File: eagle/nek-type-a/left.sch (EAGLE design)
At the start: 68 parts

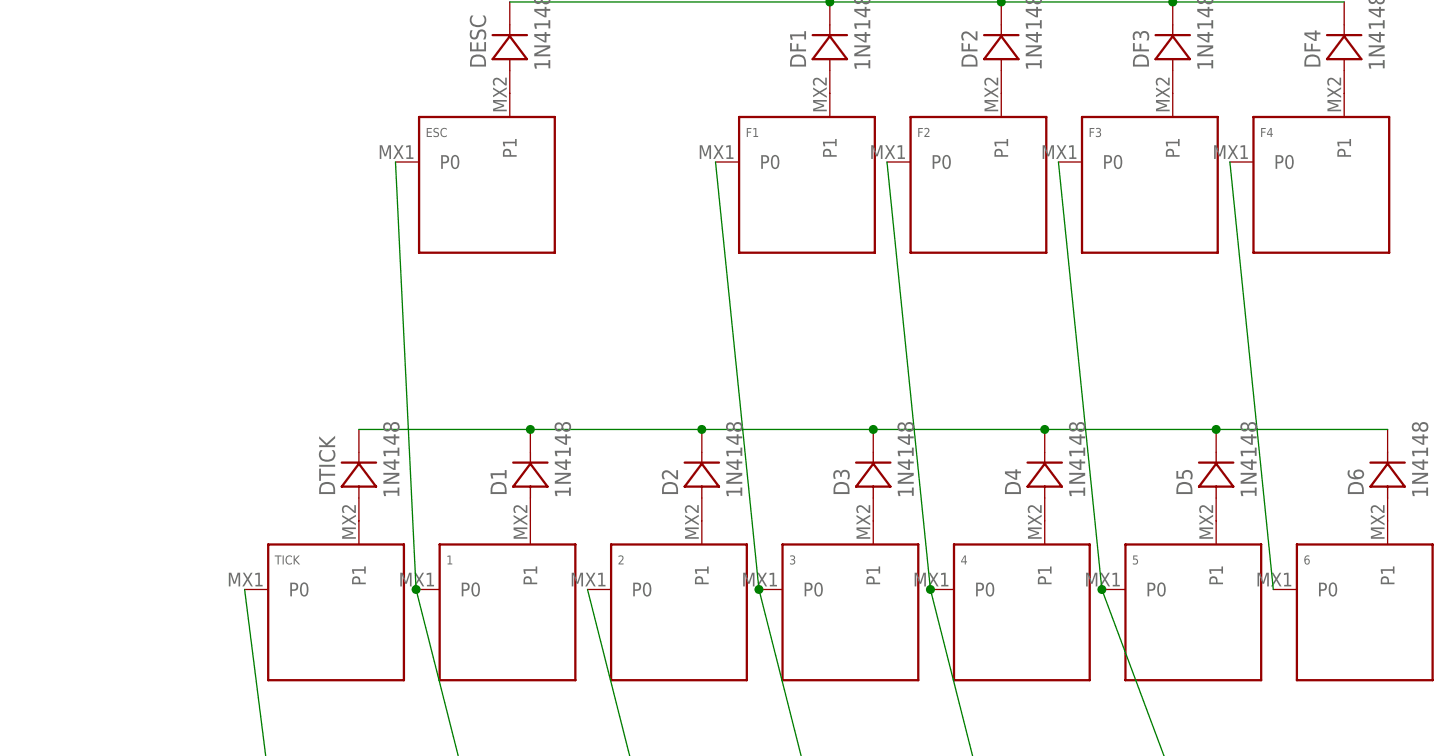
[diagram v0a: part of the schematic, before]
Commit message: columns
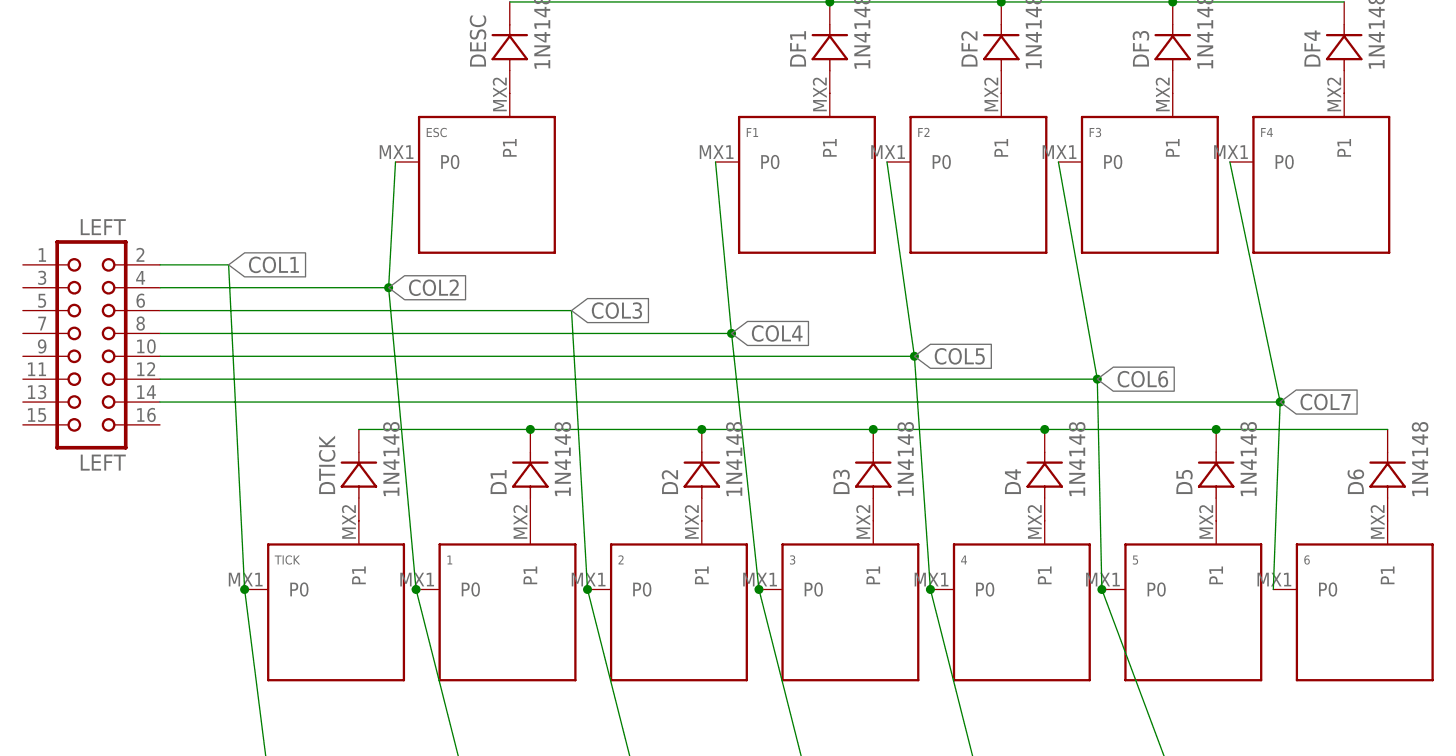
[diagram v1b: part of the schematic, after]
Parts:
- added LEFT: LEFT, con-harting:CON16
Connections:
- net ROW2.25 renamed ROW2
- removed net N$35: CAPSLOCK.P0, CONTROL.P0, SHIFT.P0, TAB.P0, TICK.P0
- removed net N$36: 1.P0, A.P0, ESC.P0, OPTION.P0, Q.P0, Z.P0
- removed net N$37: 2.P0, COMMAND.P0, S.P0, W.P0, X.P0
- removed net N$38: 3.P0, C.P0, D.P0, E.P0, F1.P0
- removed net N$39: 4.P0, F.P0, F2.P0, R.P0, SPACE.P0, V.P0
- removed net N$40: 5.P0, B.P0, F3.P0, G.P0, T.P0
- removed net N$41: 6.P0, F4.P0
- new net COL1: CAPSLOCK.P0, CONTROL.P0, LEFT.2, SHIFT.P0, TAB.P0, TICK.P0
- new net COL2: 1.P0, A.P0, ESC.P0, LEFT.4, OPTION.P0, Q.P0, Z.P0
- new net COL3: 2.P0, COMMAND.P0, LEFT.6, S.P0, W.P0, X.P0
- new net COL4: 3.P0, C.P0, D.P0, E.P0, F1.P0, LEFT.8
- new net COL5: 4.P0, F.P0, F2.P0, LEFT.10, R.P0, SPACE.P0, V.P0
- new net COL6: 5.P0, B.P0, F3.P0, G.P0, LEFT.12, T.P0
- new net COL7: 6.P0, F4.P0, LEFT.14
